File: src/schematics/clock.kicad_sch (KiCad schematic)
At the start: 2 parts, among them U7 XLH335040.000000I

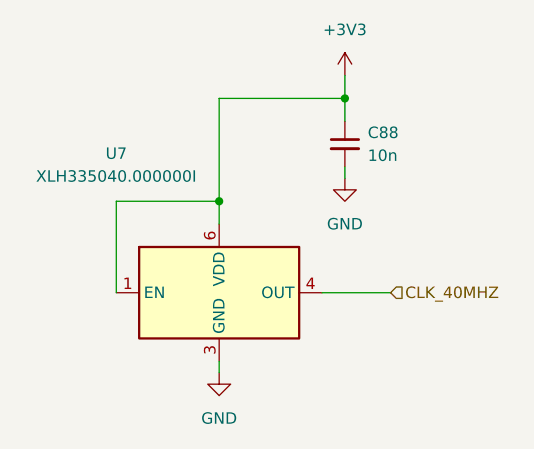
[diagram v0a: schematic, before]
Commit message: Add bom components
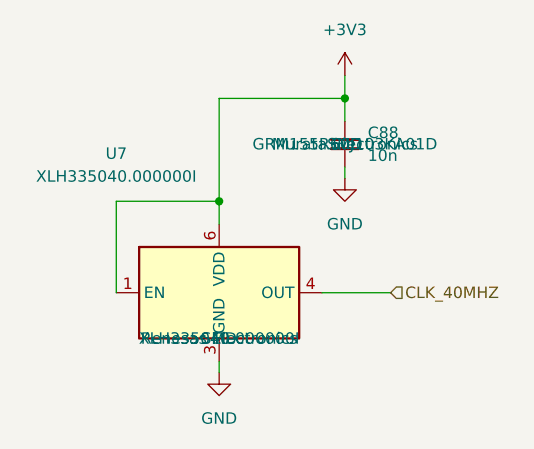
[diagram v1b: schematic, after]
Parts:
- C88: MPN (none) -> GRM155R60J103KA01D; Manufacturer (none) -> Murata Electronics; Mouting Technology (none) -> SMD
- U7: MPN (none) -> XLH335040.000000I; Manufacturer (none) -> Renesas Electronics; Mouting Technology (none) -> SMD
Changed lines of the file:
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@@
 			)
 		)
-		(property "Description" "Unpolarized capacitor, small symbol"
-			(at 168.91 76.2 0)
-			(effects
-				(font
-					(size 1.27 1.27)
-				)
-				(hide yes)
+		(property "Description" "10n 0402 X5R"
+			(at 168.91 76.2 0)
+			(effects
+				(font
+					(size 1.27 1.27)
+				)
+				(hide yes)
+			)
+		)
+		(property "Component" ""
+			(at 168.91 76.2 0)
+			(effects
+				(font
+					(size 1.27 1.27)
+				)
+			)
+		)
+		(property "MPN" "GRM155R60J103KA01D"
+			(at 168.91 76.2 0)
+			(effects
+				(font
+					(size 1.27 1.27)
+				)
+			)
+		)
+		(property "Manufacturer" "Murata Electronics"
+			(at 168.91 76.2 0)
+			(effects
+				(font
+					(size 1.27 1.27)
+				)
+			)
+		)
+		(property "Sim.Device" ""
+			(at 168.91 76.2 0)
+			(effects
+				(font
+					(size 1.27 1.27)
+				)
+			)
+		)
+		(property "Sim.Type" ""
+			(at 168.91 76.2 0)
+			(effects
+				(font
+					(size 1.27 1.27)
+				)
+			)
+		)
+		(property "Mouting Technology" "SMD"
+			(at 168.91 76.2 0)
+			(effects
+				(font
+					(size 1.27 1.27)
+				)
 			)
 		)
@@
 			)
 		)
+		(property "Component" ""
+			(at 154.94 97.79 0)
+			(effects
+				(font
+					(size 1.27 1.27)
+				)
+			)
+		)
+		(property "MPN" "XLH335040.000000I"
+			(at 154.94 97.79 0)
+			(effects
+				(font
+					(size 1.27 1.27)
+				)
+			)
+		)
+		(property "Manufacturer" "Renesas Electronics"
+			(at 154.94 97.79 0)
+			(effects
+				(font
+					(size 1.27 1.27)
+				)
+			)
+		)
+		(property "Sim.Device" ""
+			(at 154.94 97.79 0)
+			(effects
+				(font
+					(size 1.27 1.27)
+				)
+			)
+		)
+		(property "Sim.Type" ""
+			(at 154.94 97.79 0)
+			(effects
+				(font
+					(size 1.27 1.27)
+				)
+			)
+		)
+		(property "Mouting Technology" "SMD"
+			(at 154.94 97.79 0)
+			(effects
+				(font
+					(size 1.27 1.27)
+				)
+			)
+		)
